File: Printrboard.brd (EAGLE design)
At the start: 100.1 x 63 mm, 129 parts, among them J1 MICROSD, J3 USB-MICRO-PTH, J4 PCIE, Q1 RFP30N06LE, Q2 RFP30N06LE, Q3 RFP30N06LE, Q4 RFP30N06LE, U1 LM2841, U10 MCP4728, U2 A4982, U3 A4982, U4 A4982, U5 A4982, U6 AT90USB1286, U7 AP7313, U8 TXB0104, U9 PRTR5V0U4D, X1 16MHz

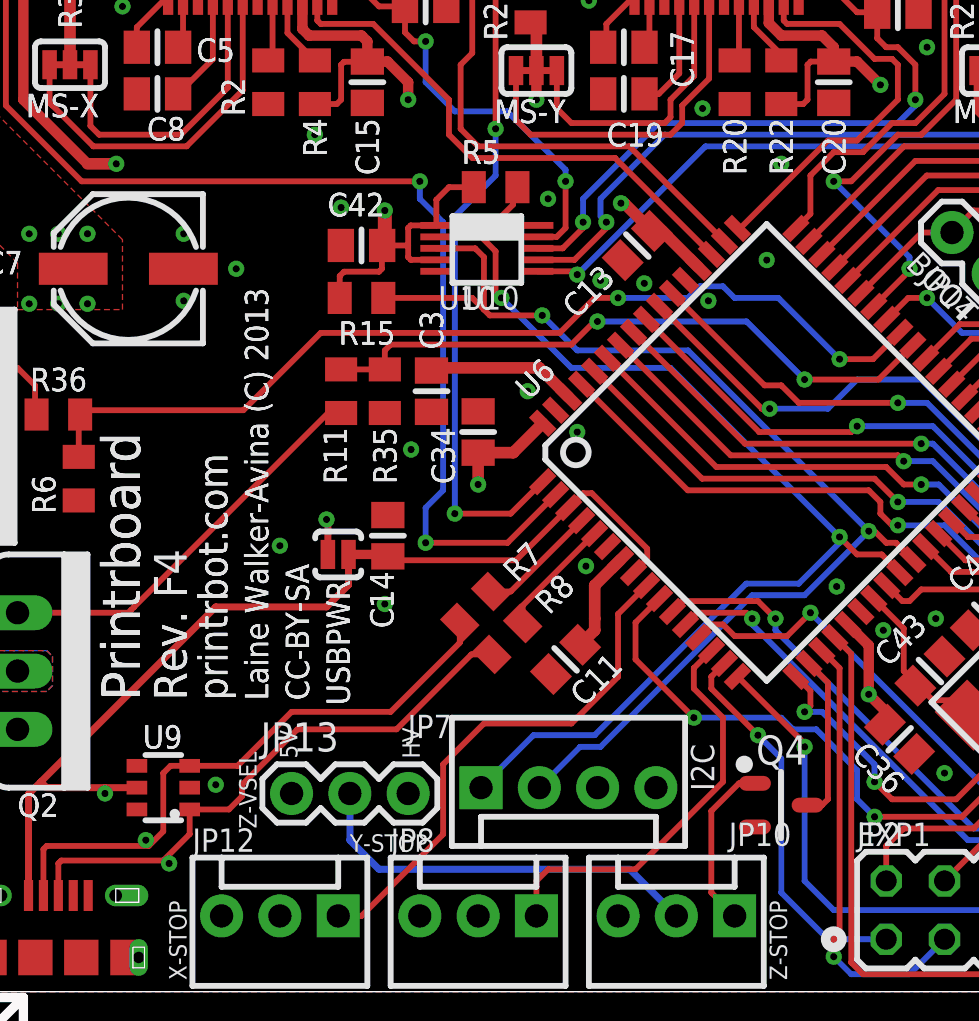
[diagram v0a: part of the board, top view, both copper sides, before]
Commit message: Bump rev to F5 and update copyright date
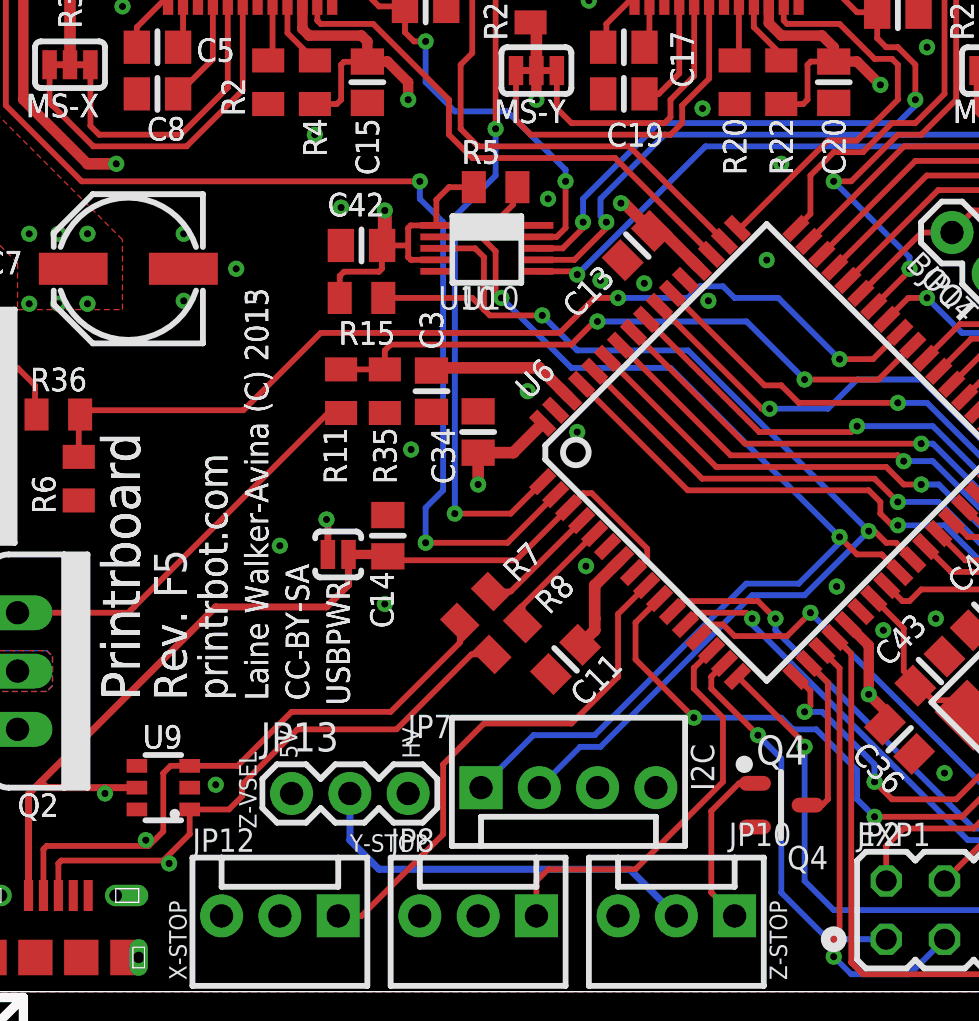
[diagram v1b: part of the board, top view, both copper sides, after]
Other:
- board text added: "Laine Walker-Avina (C) 2015"
- board text added: "Q4"
- board text added: "Rev. F5"
- board text removed: "Rev. F4"
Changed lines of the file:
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@@
 <text x="16.764" y="12.7" size="1.6764" layer="121" ratio="20" rot="R90">Printrboard</text>
 <text x="20.574" y="12.7" size="1.27" layer="121" ratio="20" rot="R90">printrbot.com</text>
-<text x="18.796" y="12.7" size="1.4224" layer="121" ratio="20" rot="R90">Rev. F4</text>
-<text x="22.352" y="12.7" size="1.016" layer="121" ratio="25" rot="R90">Laine Walker-Avina (C) 2013</text>
+<text x="18.796" y="12.7" size="1.4224" layer="121" ratio="20" rot="R90">Rev. F5</text>
+<text x="22.352" y="12.7" size="1.016" layer="121" ratio="25" rot="R90">Laine Walker-Avina (C) 2015</text>
 <text x="88.646" y="13.716" size="1.016" layer="121" ratio="25">Reset</text>
 <text x="24.13" y="12.7" size="1.016" layer="121" ratio="25" rot="R90">CC-BY-SA</text>
@@
 <wire x1="44.6913" y1="9.578009375" x2="44.6913" y2="6.677990625" width="0.254" layer="121"/>
 <circle x="43.091303125" y="9.906990625" radius="0.2499875" width="0.254" layer="121"/>
+<text x="44.958" y="5.334" size="1.016" layer="121" ratio="20">Q4</text>
 </plain>
 <attributes>
